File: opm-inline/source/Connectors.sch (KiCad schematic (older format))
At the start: 33 parts, among them J1 Info, J2 VCC_IO, J3 PWMx6, J4 Fan, J6 Current Sensing, Q7 WSD90P06DN56, U2 TerminalBlock_2_P5.08mm, U3 TerminalBlock_3_P5.08mm

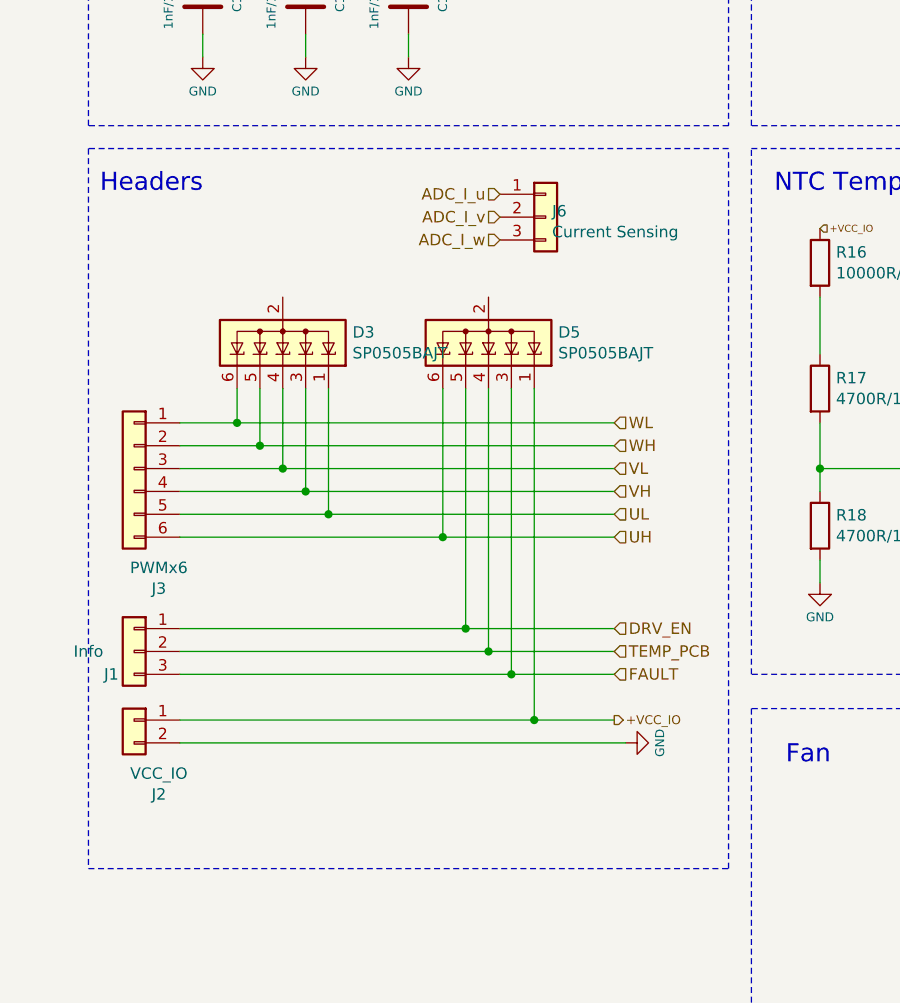
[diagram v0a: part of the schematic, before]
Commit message: more routing
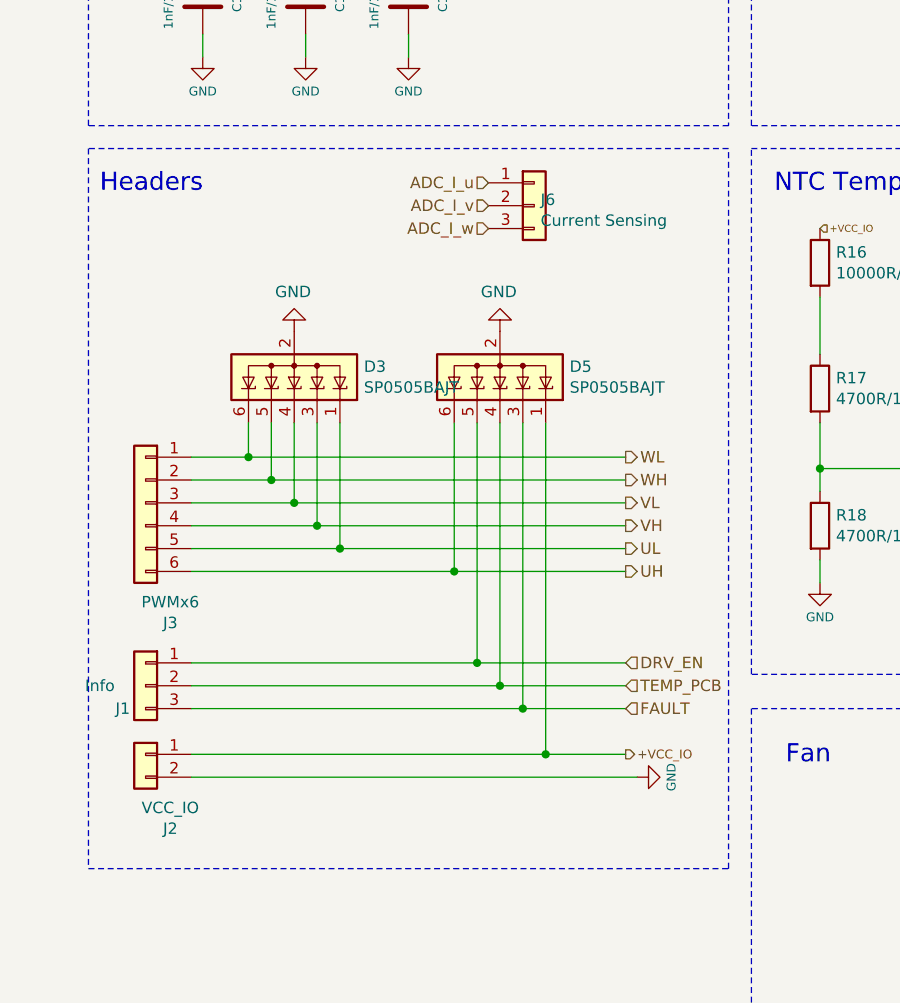
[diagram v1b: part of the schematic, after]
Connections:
- net GND: now also D3.2 (A), D5.2 (A)
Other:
- moved on the sheet: D3, D5, J1, J2, J3, J6

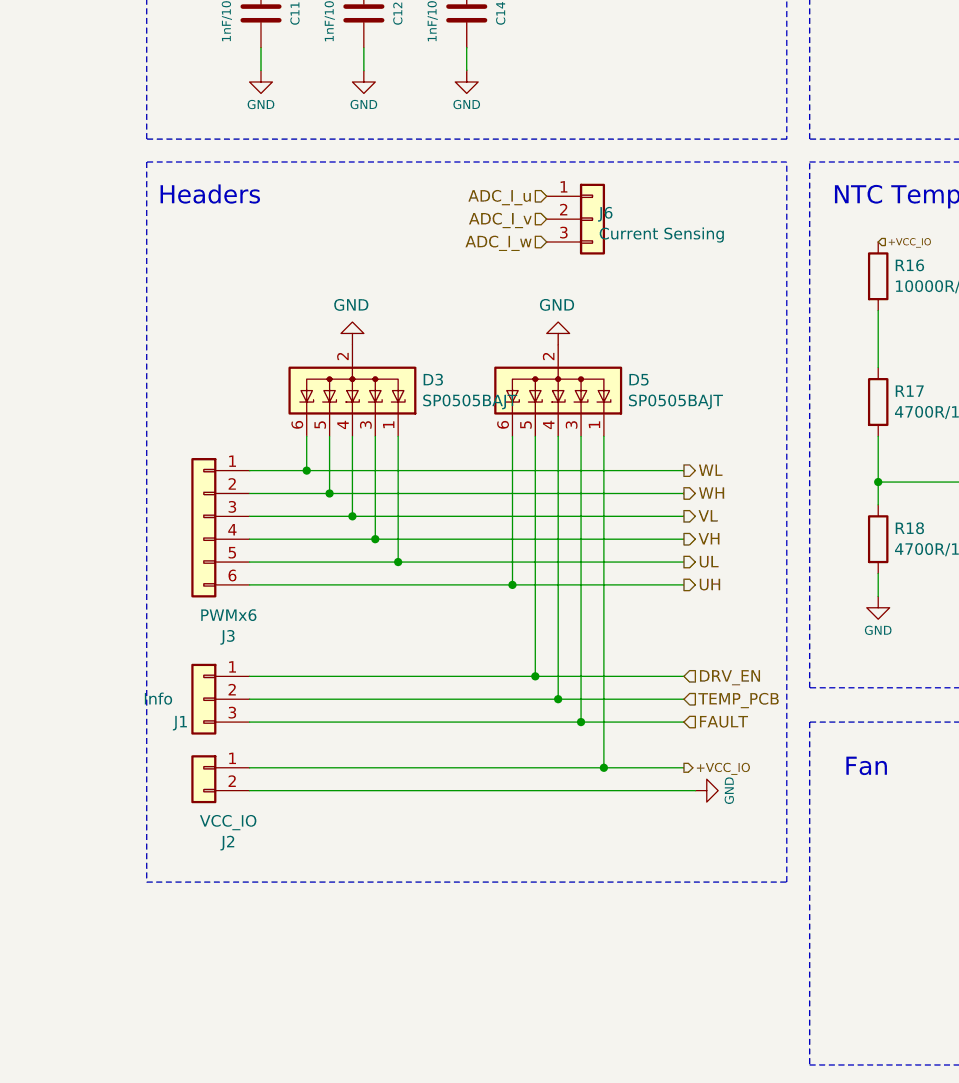
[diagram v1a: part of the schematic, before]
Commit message: esd
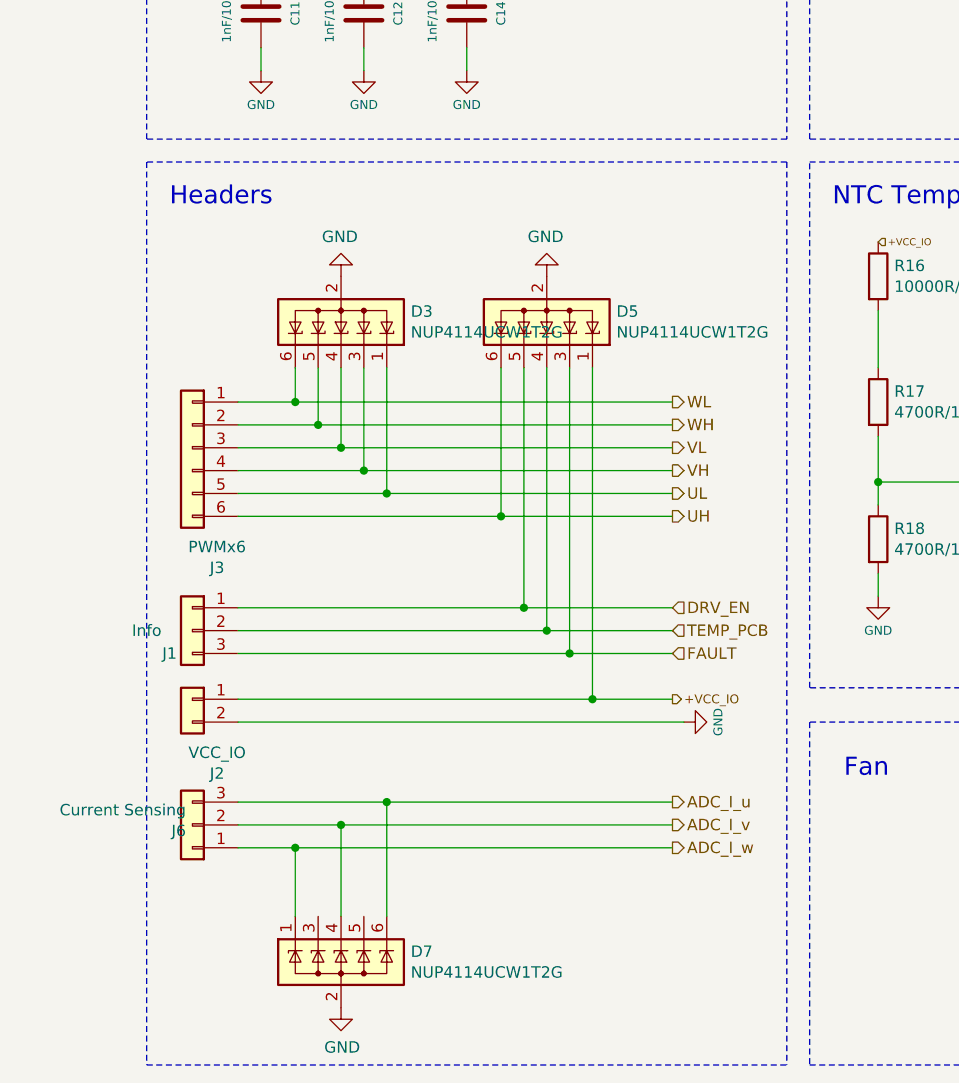
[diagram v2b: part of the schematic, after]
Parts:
- added D7: NUP4114UCW1T2G, Libraries:NUP4114UCW1T2G, symbol Power_Protection:SP0505BAJT
- D3, D5: value SP0505BAJT -> NUP4114UCW1T2G; footprint Package_TO_SOT_SMD:SOT-363_SC-70-6 -> Libraries:NUP4114UCW1T2G; LCSC (none) -> C463643; manf_num (none) -> NUP4114UCW1T2G
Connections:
- net ADC_I_u: now also J6.3 (Pin_3), D7.6 (K); no longer J6.1 (Pin_1)
- net ADC_I_v: now also D7.4 (K)
- net ADC_I_w: now also J6.1 (Pin_1), D7.1 (K); no longer J6.3 (Pin_3)
- net GND: now also D7.2 (A)
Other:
- moved on the sheet: D3, D5, J1, J2, J3, J6
